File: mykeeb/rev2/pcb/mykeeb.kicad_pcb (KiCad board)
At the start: 2 copper layers, 158.4 x 133.3 mm, 104 parts, among them K0 KEYSW, K1 KEYSW, K10 KEYSW, K11 KEYSW, K12 KEYSW, K13 KEYSW, K14 KEYSW, K15 KEYSW, K16 KEYSW, K2 KEYSW, K20 KEYSW, K21 KEYSW, K22 KEYSW, K23 KEYSW, K24 KEYSW, K25 KEYSW, K26 KEYSW, K3 KEYSW, K30 KEYSW, K31 KEYSW, K32 KEYSW, K33 KEYSW, K34 KEYSW, K35 KEYSW, K36 KEYSW, K4 KEYSW, K42 KEYSW, K43 KEYSW, K44 KEYSW, K45 KEYSW, K46 KEYSW, K5 KEYSW, K6 KEYSW, SW1 SW_Push, U1 ProMicro

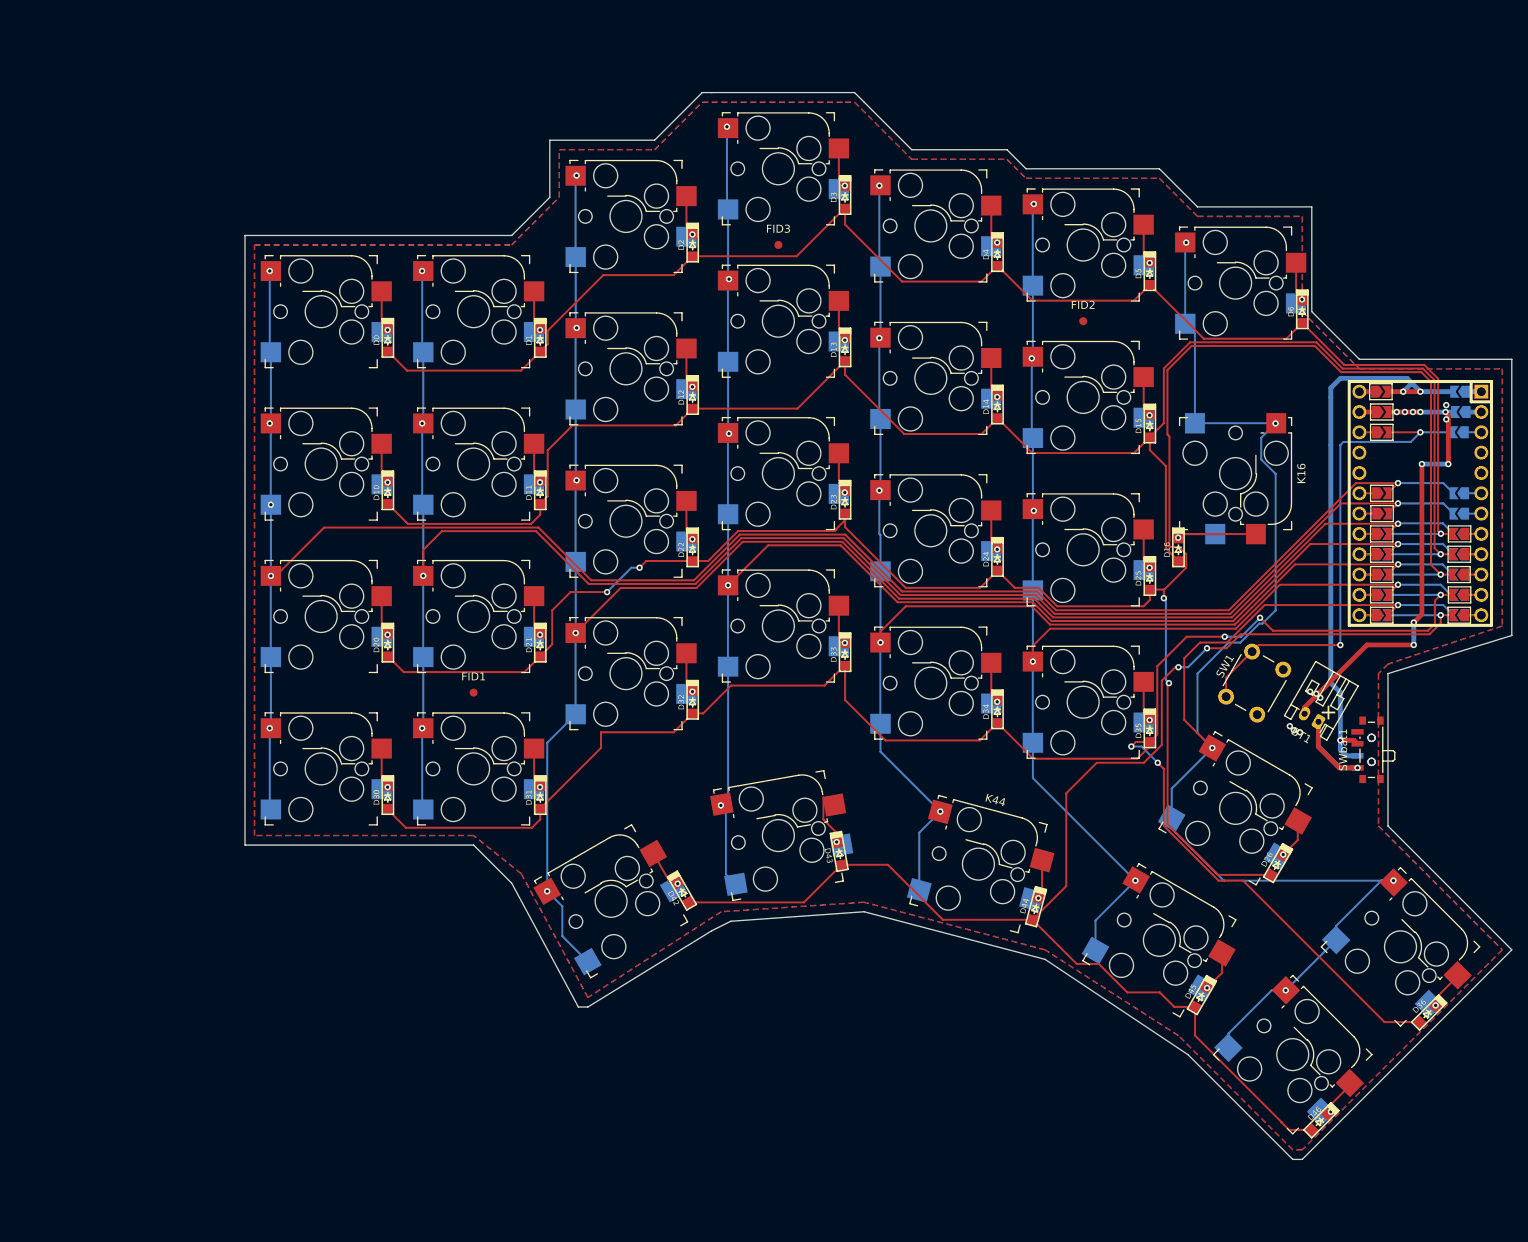
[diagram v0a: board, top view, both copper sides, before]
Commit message: wip
Signed-off-by: Maximilian Huber <gh@maxhbr.de>
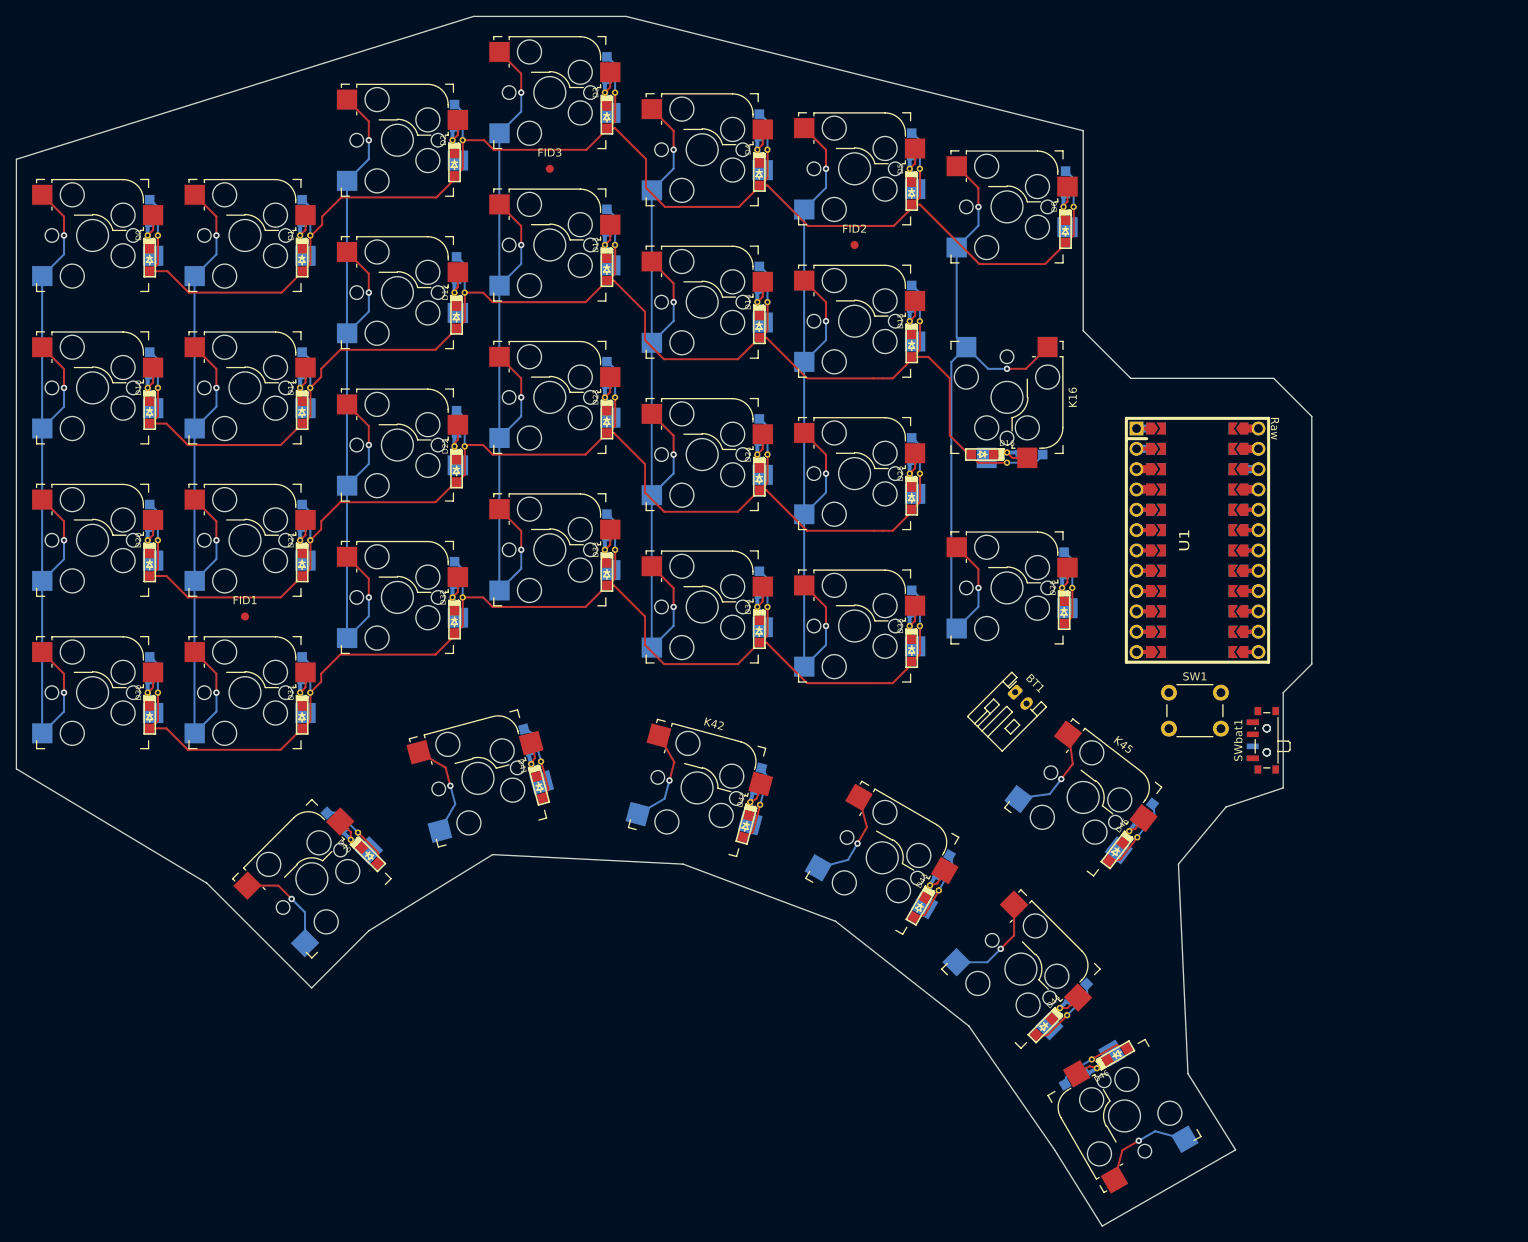
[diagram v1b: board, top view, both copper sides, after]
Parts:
- removed D36: DIODE, Keebio-Parts:D_SOD123F
- removed JPbat+a0, JPbat+b0, JPc0a1, JPc0b1, JPc1a1, JPc1b1, JPc2a1, JPc2b1, JPc3a1, JPc3b1, JPc4a1, JPc4b1, JPc5a1, JPc5b1, JPc6a1, JPc6b1, JPgbda0, JPgndb0, JPr0a1, JPr0b1, JPr1a1, JPr1b1, JPr2a1, JPr2b1, JPr3a1, JPr3b1, JPr4a1, JPr4b1, JPresa0, JPresb0: SolderJumper_2_Open, Jumper:SolderJumper-2_P1.3mm_Open_TrianglePad1.0x1.5mm
- removed K36: KEYSW, mykeeb:Kailh_socket_MX_reversible_1u
- added D40: DIODE, mykeeb:my_dual_D_SOD123F_v2, F.Cu at (59.8, 123.0)
- added D41: DIODE, mykeeb:my_dual_D_SOD123F_v2, F.Cu at (82.5, 113.6)
- added K40: KEYSW, mykeeb:Kailh_socket_MX_reversible_1u, F.Cu at (54.8, 128.0)
- added K41: KEYSW, mykeeb:Kailh_socket_MX_reversible_1u, F.Cu at (75.6, 115.5)
- D0, D1, D10, D11, D12, D13, D14, D15, D16, D2, D20, D21, D22, D23, D24, D25, D26, D3, D30, D31, D32, D33, D34, D35, D4, D42, D43, D44, D45, D46, D5, D6: footprint Keebio-Parts:D_SOD123F -> mykeeb:my_dual_D_SOD123F_v2
- K42: footprint mykeeb:Kailh_socket_MX_reversible_1u -> mykeeb:Kailh_socket_MX_reversible_1.25u
- K44: footprint mykeeb:Kailh_socket_MX_reversible_1.25u -> mykeeb:Kailh_socket_MX_reversible_1u
- K45: footprint mykeeb:Kailh_socket_MX_reversible_1u -> mykeeb:Kailh_socket_MX_reversible_1.5u
- U1: footprint Keebio-Parts:ArduinoProMicro-BackSide -> mykeeb:my_reversible_Pro_Micro; moved to F.Cu
- moved D26 43.7 mm to (148.8, 91.7), turned to -90 degrees
- moved K26 39.7 mm to (141.7, 91.7), turned to 0 degrees
- moved BT1 38.1 mm to (142.7, 104.7), turned to -45 degrees
- moved D20 32.5 mm to (34.5, 85.7)
- moved D21 32.5 mm to (53.6, 85.7)
- moved D23 32.5 mm to (91.7, 67.9)
- moved D0 32.5 mm to (34.5, 47.6)
- moved D1 32.5 mm to (53.6, 47.6)
- moved D10 32.5 mm to (34.5, 66.7)
- moved D11 32.5 mm to (53.6, 66.7)
- moved D13 32.5 mm to (91.7, 48.8)
- moved D14 32.5 mm to (110.7, 56.0)
- moved D15 32.5 mm to (129.8, 58.3)
- moved D2 32.5 mm to (72.6, 35.7)
- moved D24 32.5 mm to (110.7, 75.0)
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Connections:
- U1 pad 1: b0b -> unconnected-(U1-Pad1)
- U1 pad 10: c4b -> row2
- U1 pad 11: c5b -> row3
- U1 pad 12: c6b -> row4
- U1 pad 13: c6a -> col6
- U1 pad 14: c5a -> col5
- U1 pad 15: c4a -> col4
- U1 pad 16: c3a -> col3
- U1 pad 17: c2a -> col2
- U1 pad 18: c1a -> col1
- U1 pad 19: c0a -> col0
- U1 pad 2: g0b -> unconnected-(U1-Pad2)
- U1 pad 22: rst0a -> RST
- U1 pad 23: g0a -> GND
- U1 pad 24: b0a -> Bat+
- U1 pad 3: rst0b -> GND
- U1 pad 4: unconnected-(U1-Pad4) -> GND
- U1 pad 6: c0b -> unconnected-(U1-Pad6)
- U1 pad 7: c1b -> unconnected-(U1-Pad7)
- U1 pad 8: c2b -> row0
- U1 pad 9: c3b -> row1
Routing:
- net row4: track 182.8 -> 0.00 mm, vias 3 -> 0
- net row2: track 262.7 -> 111.3 mm, vias 5 -> 0
- net row3: track 234.2 -> 111.3 mm, vias 5 -> 0
- net col0: track 236.0 -> 119.2 mm, vias 6 -> 5
- net col2: track 227.7 -> 119.2 mm, vias 6 -> 5
- net col6: track 206.6 -> 99.0 mm, vias 6 -> 4
- net col1: track 217.7 -> 119.2 mm
- net row1: track 210.9 -> 127.9 mm, vias 1 -> 0
- net col3: track 199.5 -> 119.2 mm, vias 6 -> 5
- net Bat+: track 72.6 -> 0.00 mm, vias 3 -> 0
- net RST: track 62.2 -> 0.00 mm, vias 2 -> 0
- net GND: track 58.9 -> 0.00 mm, vias 17 -> 0
- net col4: track 173.3 -> 119.2 mm, vias 6 -> 5
- net row0: track 184.4 -> 134.7 mm, vias 1 -> 0
- net col5: track 161.0 -> 119.2 mm, vias 6 -> 5
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- removed copper zone on B.Cu, net GND
- removed copper zone on F.Cu, net GND
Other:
- board size 158.4 x 133.3 mm -> 161.9 x 151.2 mm
- board text removed: "+"
